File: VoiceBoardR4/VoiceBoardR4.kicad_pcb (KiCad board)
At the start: 4 copper layers, 130 x 49.9 mm, 179 parts, among them Q201 BC857, Q202 BC857, Q301 BC857, Q302 BC857, Q401 BC857, Q402 BC857, Q403 BC847, Q404 BC857, Q405 BC847, Q406 BC857, U101 TMUX4053, U102 TMUX4053, U103 VoiceBoardConn_18P_254P, U201 TL074, U202 TL074, U203 MCP4451-104E-ST, U204 TL074, U205 MCP4451-104E-ST, U206 TL074, U301 TL074, U302 AD5280, U303 LM13700, U304 DI79L05ZAB, U305 DI78L05ZAB, U402 LM13700, U403 TL074, U404 TL074

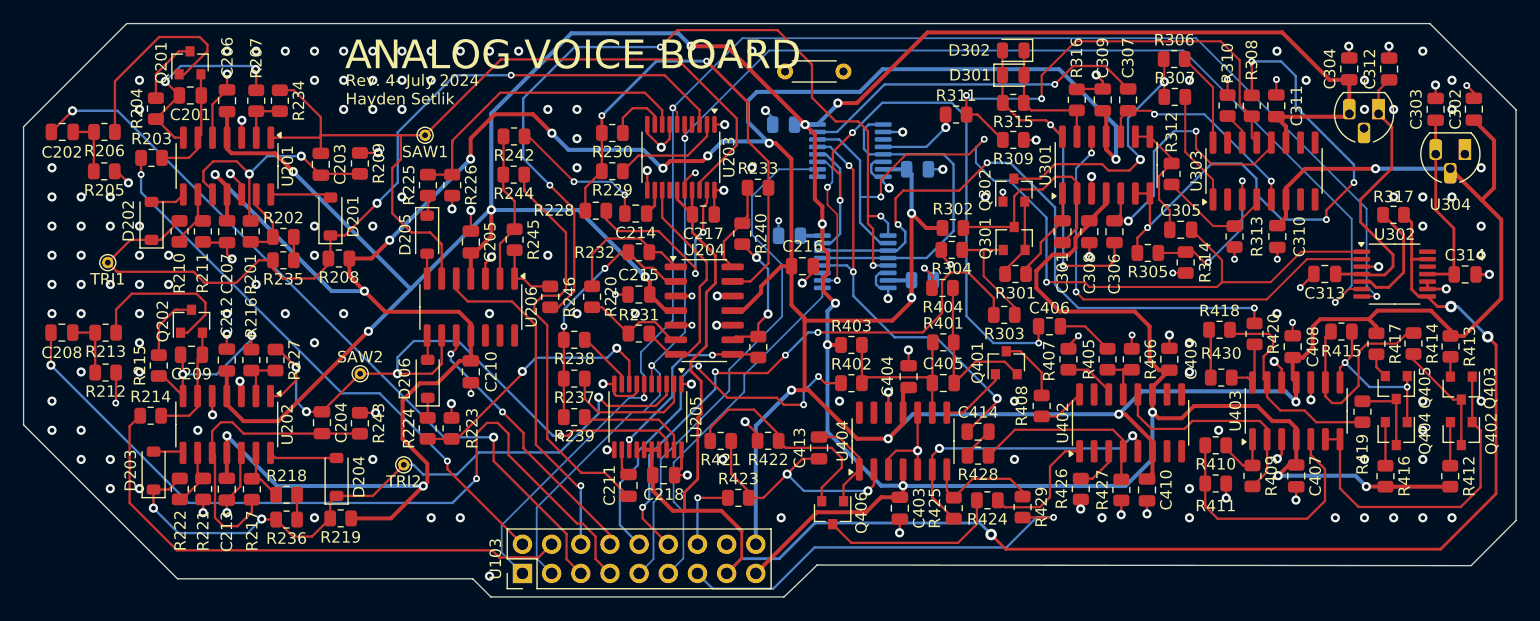
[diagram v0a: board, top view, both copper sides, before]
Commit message: voice rev4 passing DRC
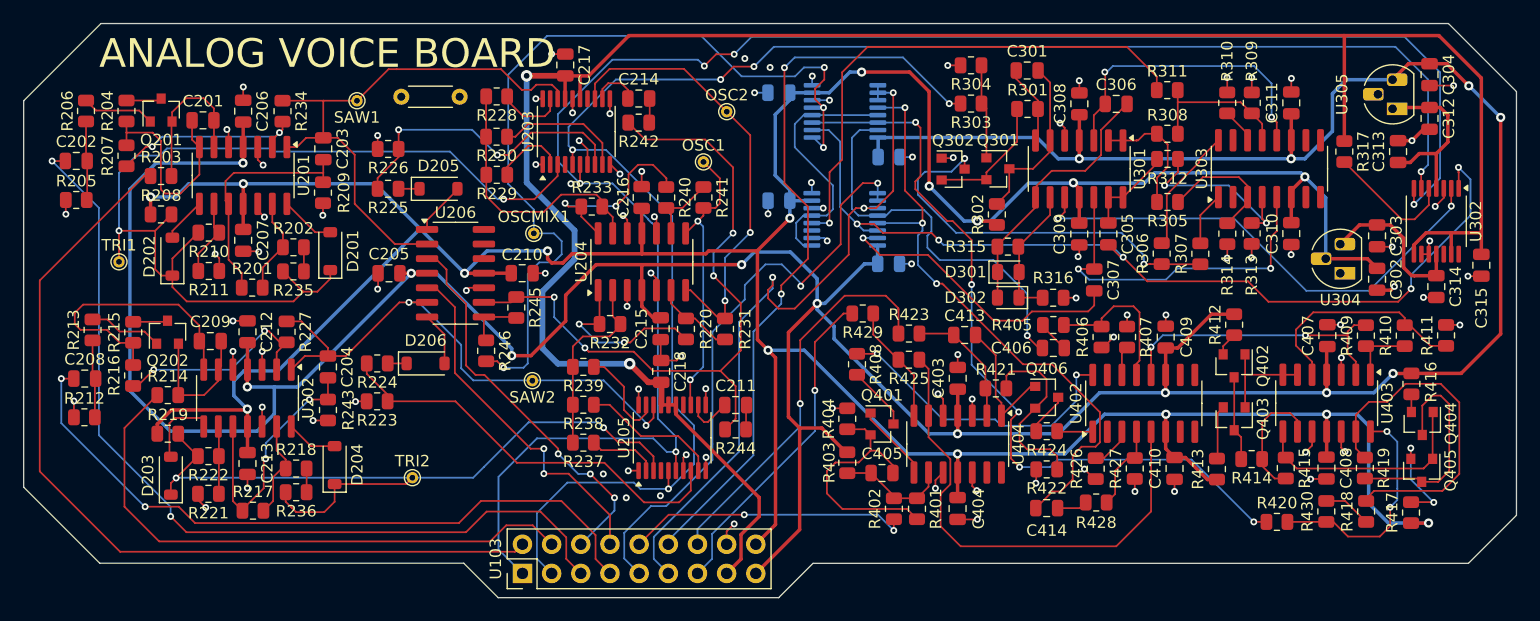
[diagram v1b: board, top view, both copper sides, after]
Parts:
- added C315: 100n, Capacitor_SMD:C_0805_2012Metric, F.Cu at (126.9, 21.1)
- added OSC1: OSC1, TestPoint:TestPoint_THTPad_D1.0mm_Drill0.5mm, F.Cu at (59.2, 12.1)
- added OSC2: OSC2, TestPoint:TestPoint_THTPad_D1.0mm_Drill0.5mm, F.Cu at (61.2, 7.67)
- added OSCMIX1: OSC2, TestPoint:TestPoint_THTPad_D1.0mm_Drill0.5mm, F.Cu at (44.4, 18.3)
- R225: value 92k -> 100k
- R226: value 100k -> 47k
- R245: value 56k -> 33k
- moved R247 33.5 mm to (32.9, 6.38)
- moved R244 29.4 mm to (62.0, 35.3)
- moved R421 24.4 mm to (84.7, 31.8), turned to 0 degrees
- moved R422 24.4 mm to (89.1, 38.8)
- moved R411 23.8 mm to (123.9, 27.2), turned to 90 degrees
- moved R412 23.0 mm to (105.4, 26.2), turned to 90 degrees
- moved R413 23.0 mm to (103.9, 38.8), turned to 90 degrees
- moved R429 21.9 mm to (73.1, 25.2), turned to 180 degrees
- moved D302 21.5 mm to (85.7, 23.9)
- moved Q406 21.2 mm to (89.1, 32.5), turned to 0 degrees
- moved R309 21.0 mm to (107.0, 6.91), turned to -90 degrees
- moved Q402 20.6 mm to (105.4, 29.8)
- moved R423 20.6 mm to (77.1, 27.0)
- moved R418 20.3 mm to (116.9, 42.5), turned to 90 degrees
- moved Q403 20.0 mm to (105.4, 34.4)
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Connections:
- net Net-(U203A-P0B) renamed /DCO/O2_MIXF
- net Net-(U205A-P0B) renamed /DCO/O1_MIXF
- C305 pad 1: Net-(U301C--) -> Net-(U301D--)
- C306 pad 1: Net-(U301B-+) -> Net-(U301A-+)
- C307 pad 1: Net-(U301C-+) -> Net-(U301D-+)
- R242 pad 2: Net-(U206A--) -> Net-(U206C--)
- R244 pad 2: Net-(U206A--) -> Net-(U206C--)
- R245 pad 1: Net-(U206A--) -> Net-(U206C--)
- R305 pad 2: Net-(U301B--) -> Net-(U301A--)
- R308 pad 2: Net-(U301B--) -> Net-(U301A--)
- R312 pad 2: Net-(U301C--) -> Net-(U301D--)
- U206 pad 1: Net-(R245-Pad2) -> Net-(D205-A)
- U206 pad 10: PWM_2_CV -> GND
- U206 pad 2: Net-(U206A--) -> SAW1_FULL
- U206 pad 3: GND -> PWM_1_CV
- U206 pad 5: PWM_1_CV -> PWM_2_CV
- U206 pad 6: SAW1_FULL -> SAW2_FULL
- U206 pad 7: Net-(D205-A) -> Net-(D206-A)
- U206 pad 8: Net-(D206-A) -> Net-(R245-Pad2)
- U206 pad 9: SAW2_FULL -> Net-(U206C--)
- U301 pad 1: Net-(C301-Pad1) -> Net-(U301A--)
- U301 pad 13: Net-(D301-A) -> Net-(U301D--)
- U301 pad 14: Net-(D301-K) -> Net-(U301D--)
- U301 pad 2: Net-(Q301-C) -> Net-(U301A--)
- U301 pad 3: GND -> Net-(U301A-+)
- U301 pad 5: Net-(U301B-+) -> GND
- U301 pad 6: Net-(U301B--) -> Net-(Q301-C)
- U301 pad 7: Net-(U301B--) -> Net-(C301-Pad1)
- U301 pad 8: Net-(U301C--) -> Net-(D301-K)
- U301 pad 9: Net-(U301C--) -> Net-(D301-A)
- U302 pad 2: Net-(U301D-+) -> Net-(U301C-+)
- U303 pad 12: Net-(U301B-+) -> Net-(U301A-+)
- U303 pad 5: Net-(U301C-+) -> Net-(U301D-+)
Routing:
- net Net-(U206C--): track 0.00 -> 61.4 mm, vias 0 -> 4
- net -12V: track 382.4 -> 323.6 mm, vias 18 -> 16
- net Net-(U301B--): track 50.8 -> 0.00 mm, vias 4 -> 0
- net LP_IN: track 7.28 -> 45.7 mm
- net Net-(C211-Pad2): track 36.1 -> 2.14 mm
- net SDA: track 129.7 -> 160.4 mm, vias 3 -> 5
- net +3.3V: track 153.7 -> 184.0 mm, vias 3 -> 2
- net Net-(U303A--): track 41.4 -> 13.4 mm, vias 2 -> 0
- net VCA_CV: track 6.68 -> 34.3 mm
- net SAW1_FULL: track 76.3 -> 49.1 mm
- net Net-(U301A-+): track 0.00 -> 26.9 mm, vias 0 -> 2
- net LEVEL_1_CV: track 49.3 -> 75.2 mm, vias 2 -> 0
- net Net-(U301B-+): track 24.9 -> 0.00 mm, vias 2 -> 0
- net Net-(U301C-+): track 19.1 -> 43.6 mm
- net SCL: track 125.9 -> 148.8 mm, vias 3 -> 5
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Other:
- board size 130 x 49.9 mm -> 130 x 50 mm
